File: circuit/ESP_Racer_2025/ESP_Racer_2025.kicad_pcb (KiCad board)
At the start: 2 copper layers, 20 x 35 mm, 19 parts, among them IC1 XCL102D333CR-G, J1 Conn_LED_1, J2 Conn_LED_2, J3 Conn_Servo, U1 DRV8835DSST, U2 SFV12R-2STE1LF, U3 ESP32-C3-WROOM-02

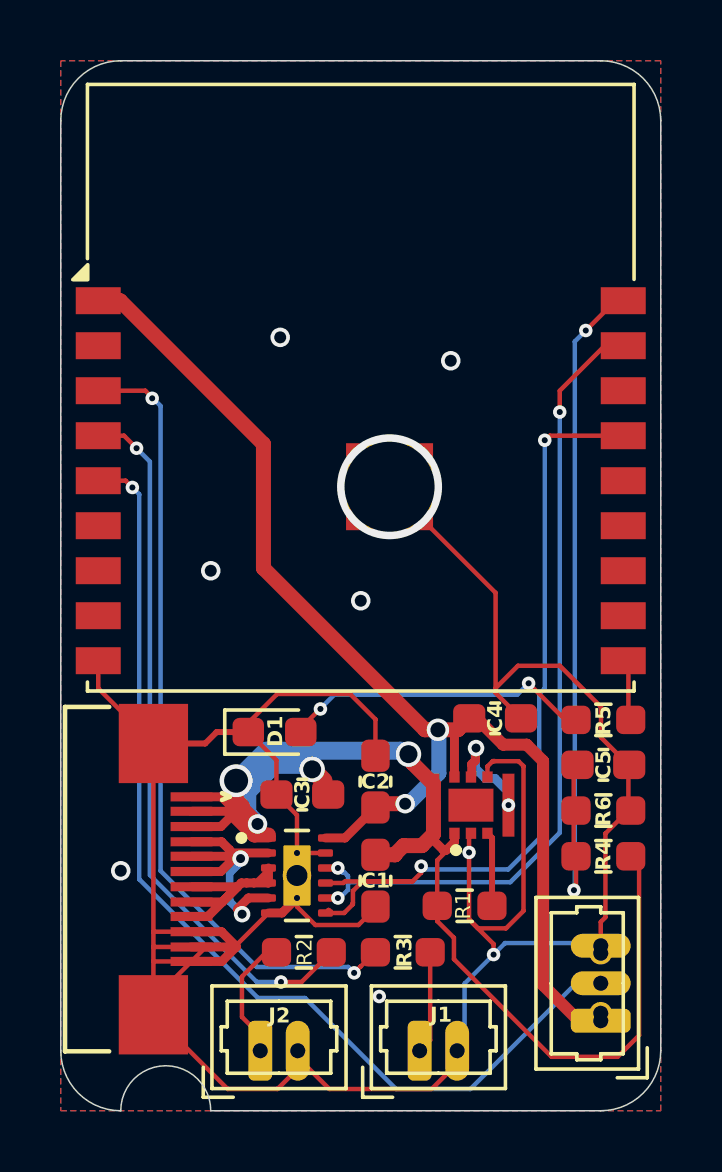
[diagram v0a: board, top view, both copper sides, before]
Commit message: fix pcb
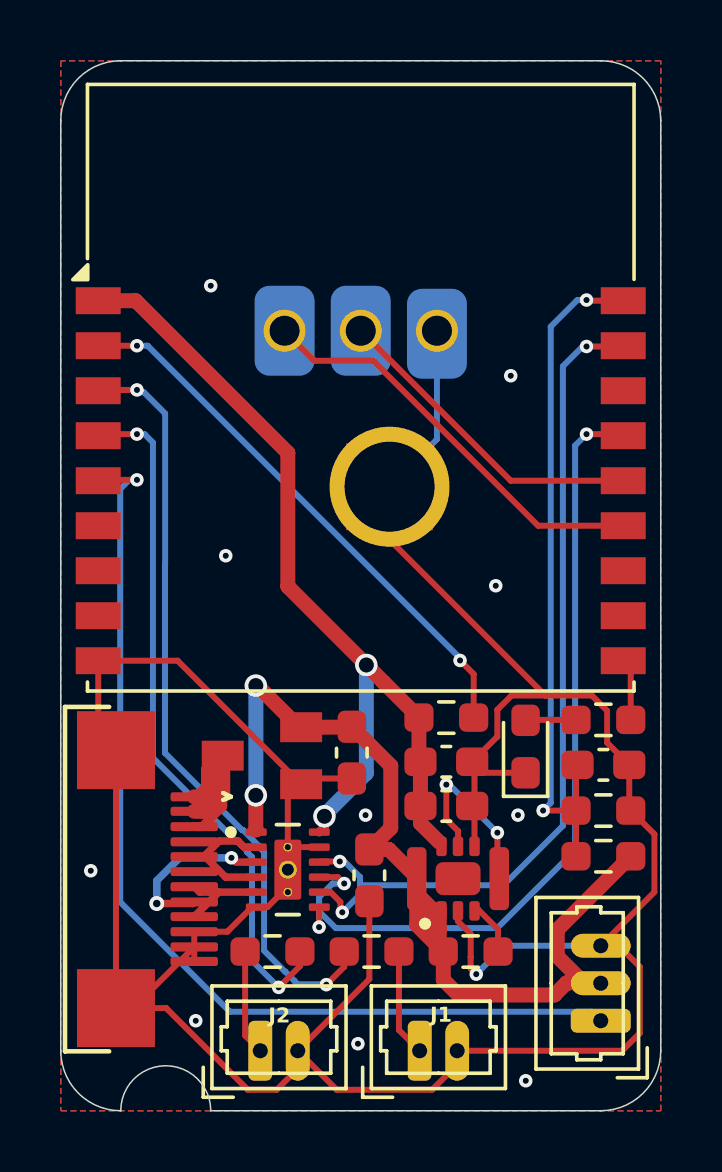
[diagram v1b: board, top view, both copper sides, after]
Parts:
- added G***: LOGO, Logo:PLEN, B.Cu at (139.0, 88.0)
- added J4: Conn_USB, Original:Serial, B.Cu at (139.0, 68.0)
- added Q3: IRLML6402, IRLML6402:SOT23, F.Cu at (135.7, 82.2)
- added R7: 10k, Resistor_SMD:R_0603_1608Metric_Pad0.98x0.95mm_HandSolder, F.Cu at (141.9, 80.9)
- C3: value 0.1u -> 10u
- C5: value 0.1μF -> 0.1u
- R2, R3: value 330 -> 300
- R5: value 330 -> 1k
- moved D1 8.38 mm to (144.5, 81.9), turned to 90 degrees
- moved C4 3.34 mm to (141.9, 83.8)
- moved C2 2.45 mm to (141.9, 82.4), turned to 0 degrees
- moved IC1 2.19 mm to (142.2, 86.3)
- moved C3 2.16 mm to (138.7, 82.1), turned to -90 degrees
- moved R1 1.54 mm to (142.7, 88.7)
- moved R2 1.05 mm to (136.1, 88.7)
- moved R3 1.04 mm to (139.4, 88.7)
- moved U1 0.36 mm to (136.6, 86.0)
- moved C1 0.27 mm to (139.3, 86.2)
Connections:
- J3 pad 1: +3.3V -> Servo_PWM
- J3 pad 2: Servo_PWM -> +BATT
- U1 pad 4: Motor_B -> Motor_A
- U1 pad 5: Motor_A -> Motor_B
- U2 pad 1: +BATT -> Net-(Q3-Pad3)
- U2 pad 2: +BATT -> Net-(Q3-Pad3)
- U2 pad 3: +BATT -> Net-(Q3-Pad3)
- U3 pad 13: unconnected-(U3-GPIO18/USB_D-Pad13) -> USB_D-
- U3 pad 14: unconnected-(U3-GPIO19/USB_D+-Pad14) -> USB_D+
- U3 pad 2: unconnected-(U3-EN-Pad2) -> Net-(U3-EN)
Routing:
- net Net-(U3-EN): track 0.00 -> 18.5 mm, vias 0 -> 2
- net USB_D-: track 0.00 -> 14.0 mm
- net +3.3V: track 41.7 -> 29.7 mm
- net USB_D+: track 0.00 -> 10.8 mm
- net +BATT: track 46.1 -> 36.1 mm, vias 4 -> 2
- net Net-(D1-A): track 10.7 -> 1.69 mm, vias 2 -> 0
- net Net-(Q3-Pad3): track 0.00 -> 8.65 mm
- net GND: track 102.6 -> 107.6 mm, vias 9 -> 11
- net Motor_A: track 9.81 -> 4.90 mm, vias 2 -> 0
- net Net-(IC1-L2): track 3.63 -> 6.09 mm
- net AIN 1: track 27.4 -> 29.4 mm
- net BATT_VCC: track 24.9 -> 23.2 mm
- net AIN 2: track 27.5 -> 29.2 mm, vias 2 -> 3
- net Motor_B: track 7.79 -> 9.10 mm, vias 0 -> 2
- net LED_1: track 26.7 -> 25.7 mm
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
